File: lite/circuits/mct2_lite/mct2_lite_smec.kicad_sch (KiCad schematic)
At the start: 1 part

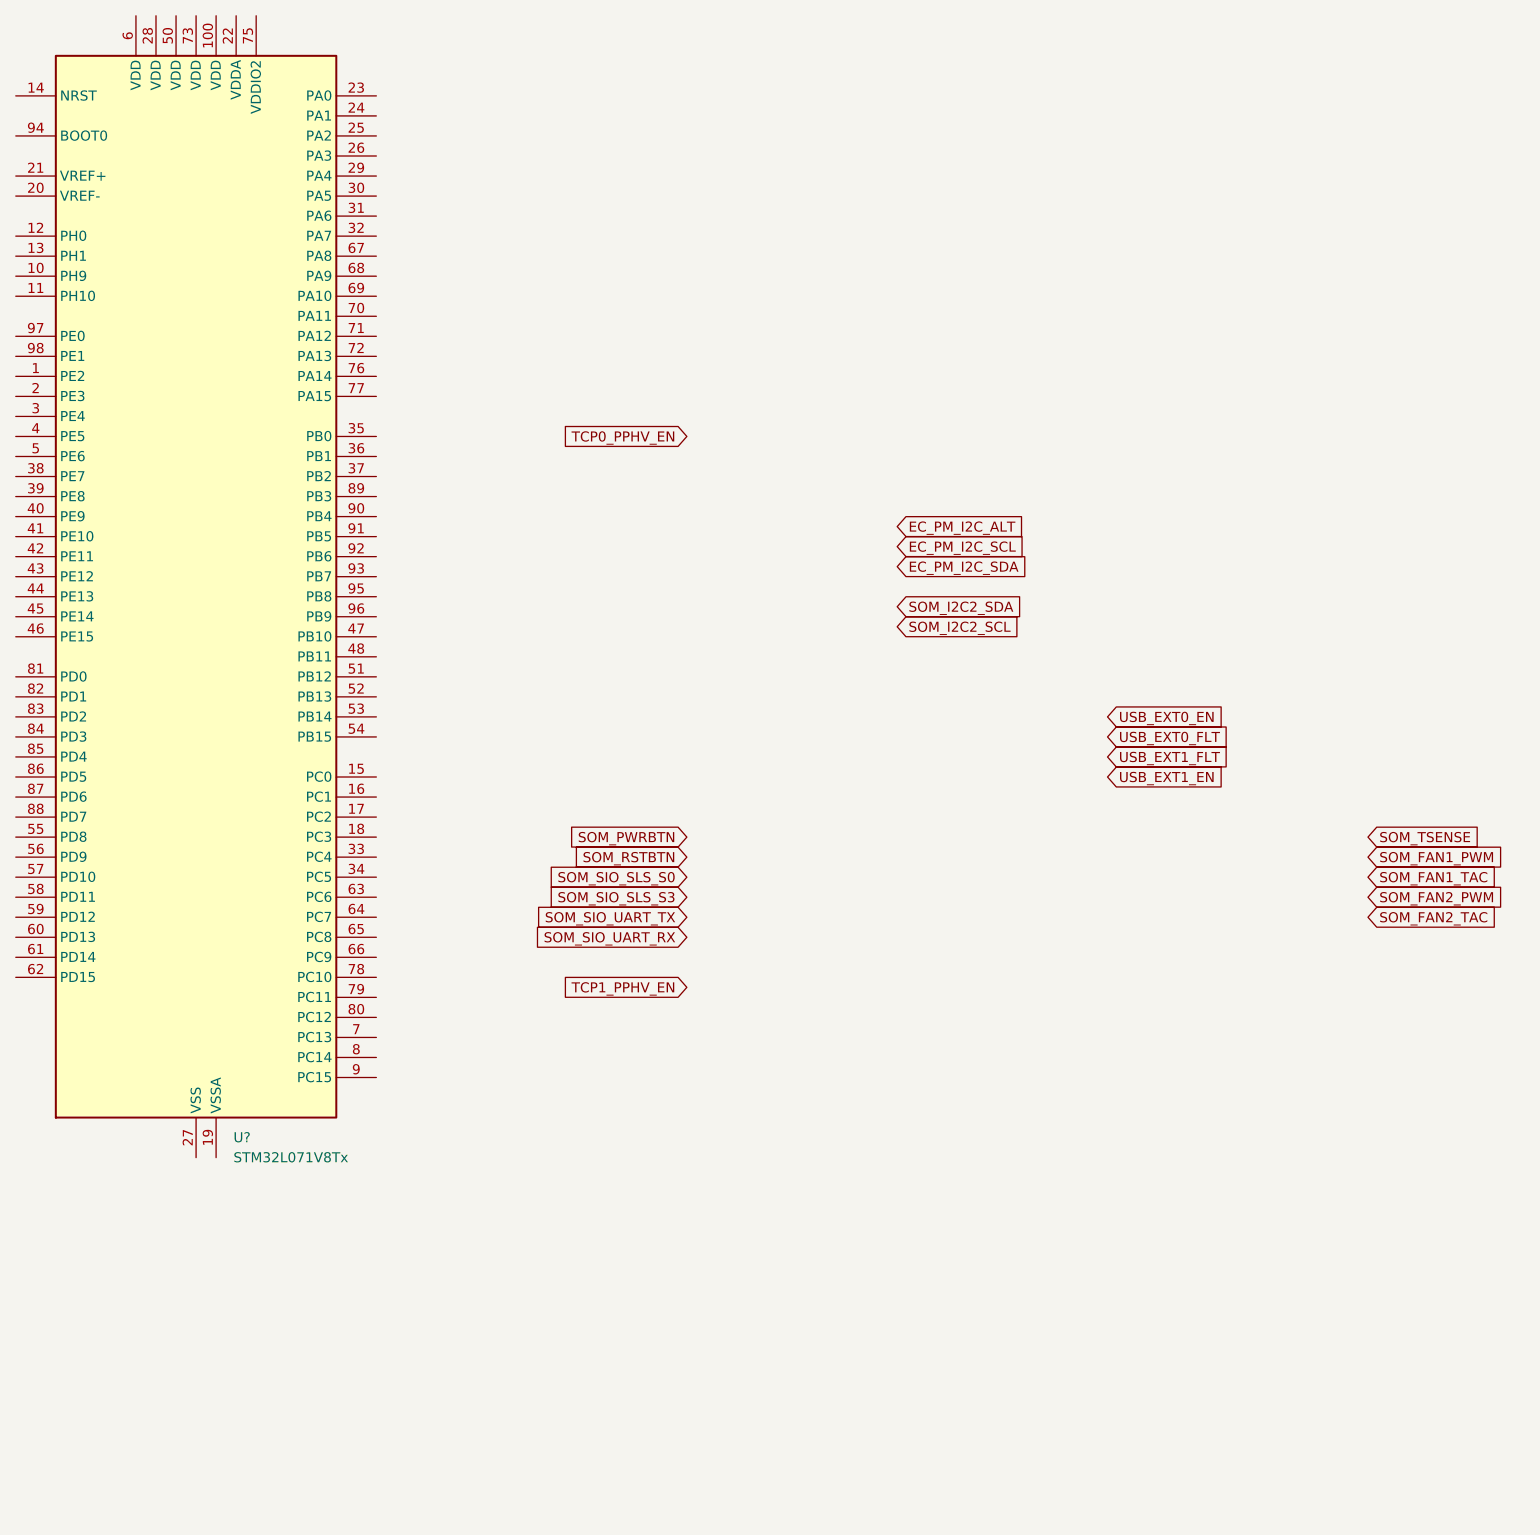
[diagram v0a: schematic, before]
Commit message: 20250529-1
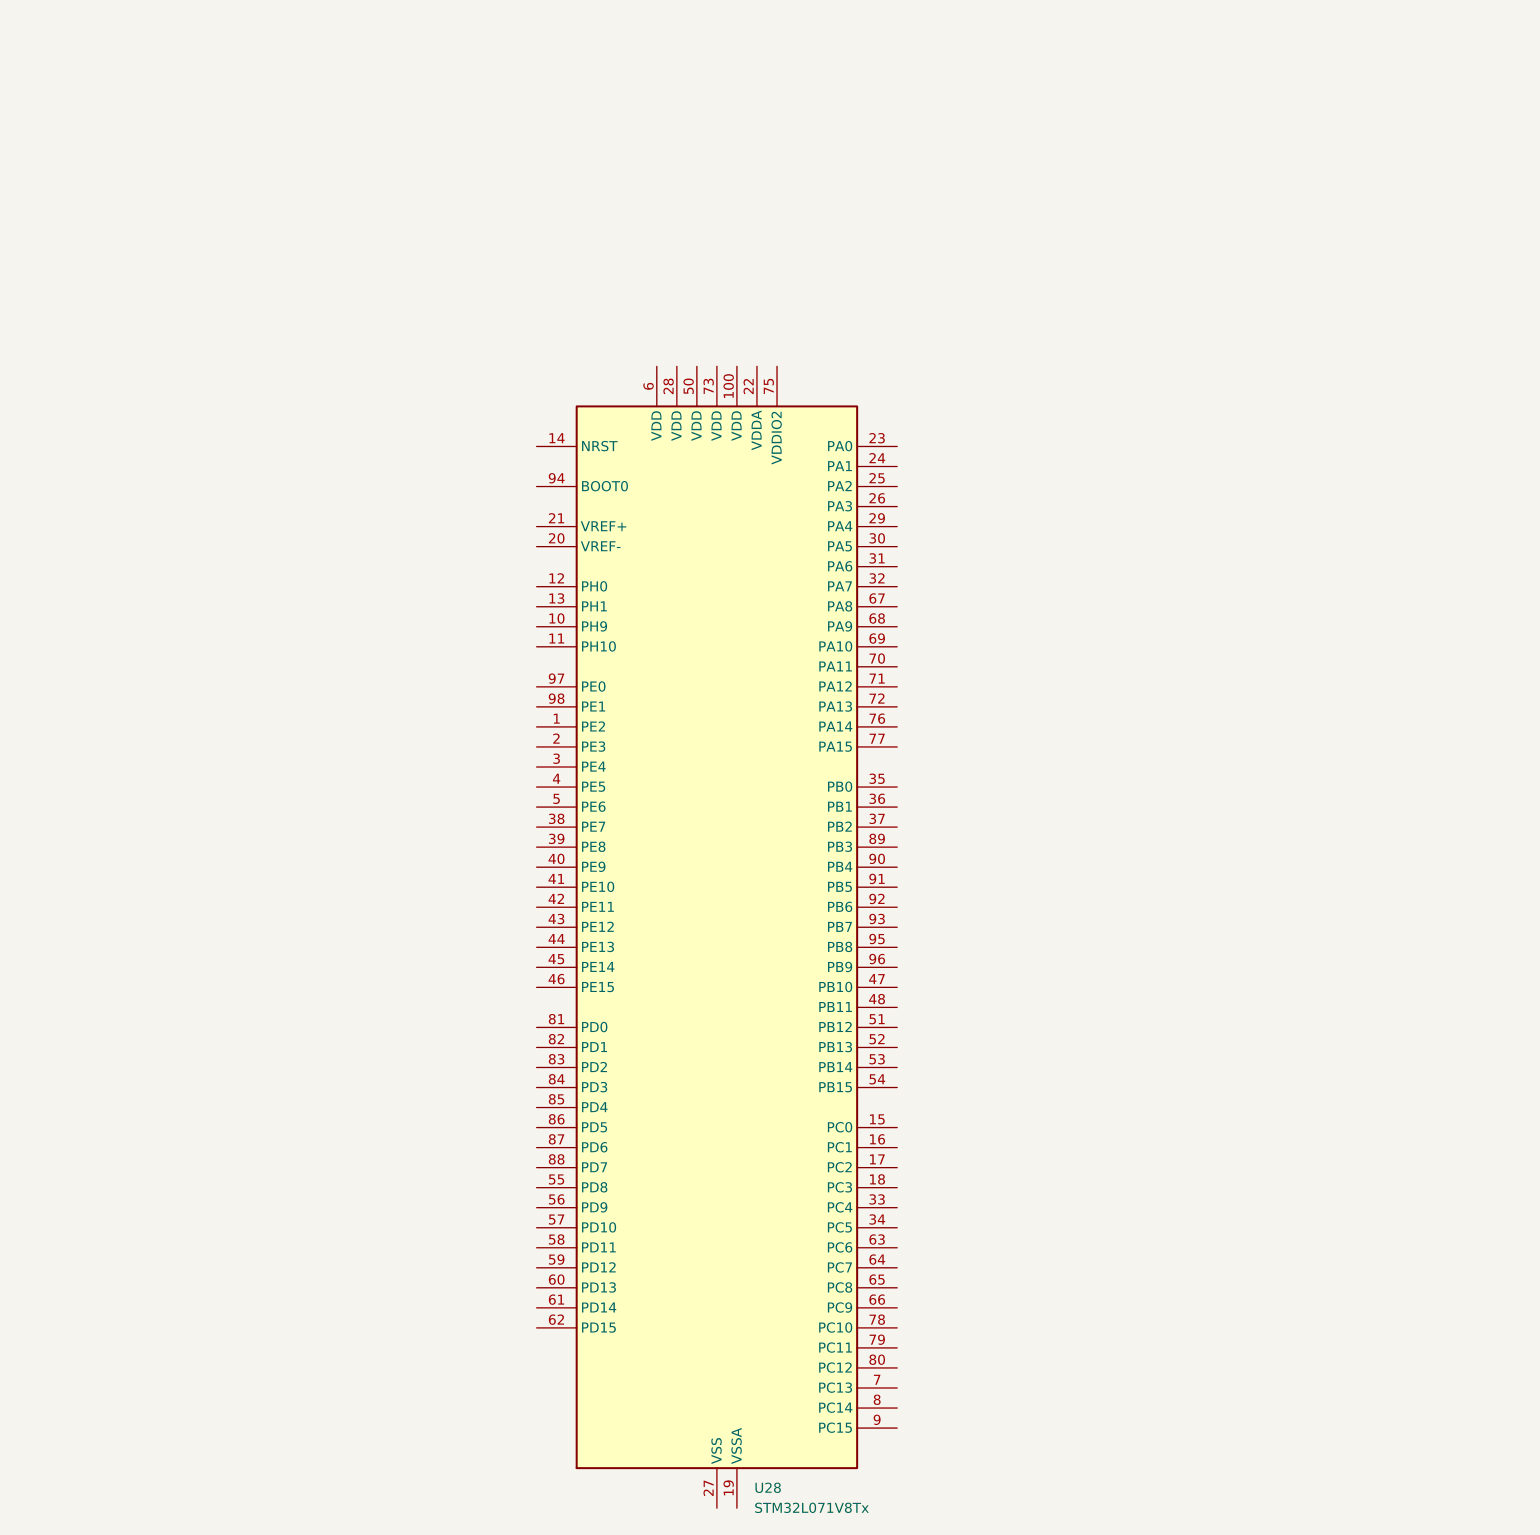
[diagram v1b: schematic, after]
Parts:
- gave numbers to parts that had none: 1
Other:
- moved on the sheet: U28
